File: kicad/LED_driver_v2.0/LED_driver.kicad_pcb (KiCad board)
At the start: 2 copper layers, 39 x 20.5 mm, 11 parts, among them J1 Conn_01x02, J2 Conn_01x02, J3 Conn_01x02, Q1 MMBT3904, Q3 2N7002

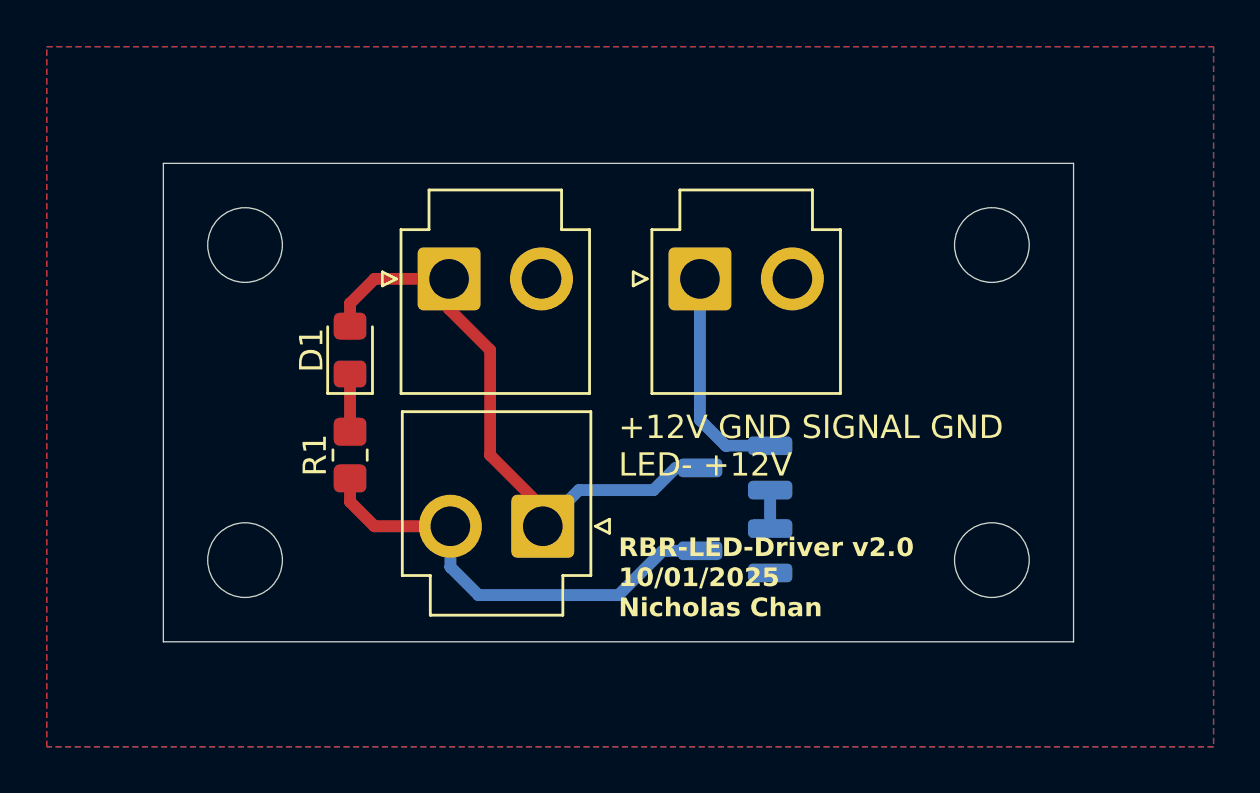
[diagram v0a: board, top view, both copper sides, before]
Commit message: nothing to do
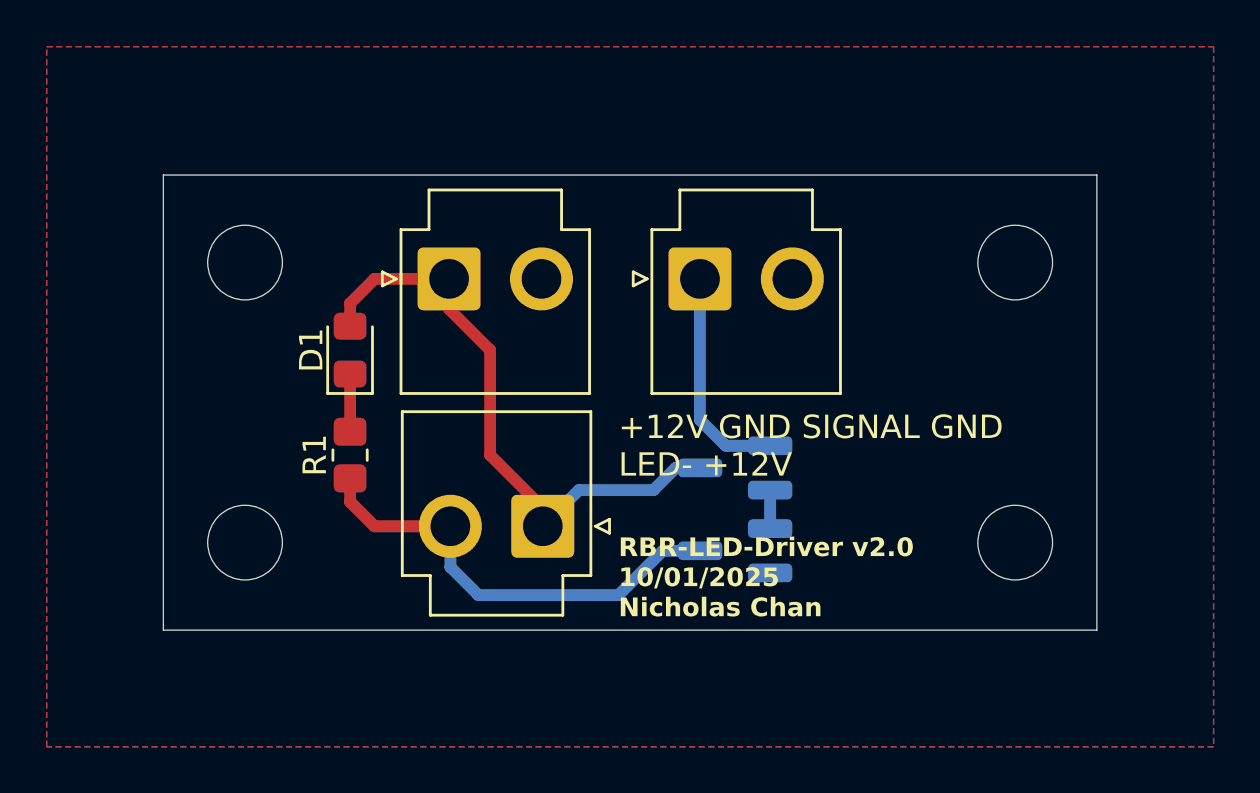
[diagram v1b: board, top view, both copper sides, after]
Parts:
- moved H2 1.25 mm to (136.5, 69.2)
- moved H4 1.25 mm to (136.5, 81.2)
- moved H1 0.75 mm to (103.5, 69.2)
- moved H3 0.75 mm to (103.5, 81.2)
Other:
- board size 39 x 20.5 mm -> 40 x 19.5 mm
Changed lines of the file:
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@@
 	(footprint "MountingHole:MountingHole_3.2mm_M3"
 		(layer "F.Cu")
-		(at 103.5 82)
+		(at 103.5 81.25)
 		(descr "Mounting Hole 3.2mm, no annular, M3")
 		(tags "mounting hole 3.2mm no annular m3")
@@
 	(footprint "MountingHole:MountingHole_3.2mm_M3"
 		(layer "F.Cu")
-		(at 103.5 68.5)
+		(at 103.5 69.25)
 		(descr "Mounting Hole 3.2mm, no annular, M3")
 		(tags "mounting hole 3.2mm no annular m3")
@@
 	(footprint "MountingHole:MountingHole_3.2mm_M3"
 		(layer "F.Cu")
-		(at 135.5 68.5)
+		(at 136.5 69.25)
 		(descr "Mounting Hole 3.2mm, no annular, M3")
 		(tags "mounting hole 3.2mm no annular m3")
@@
 	(footprint "MountingHole:MountingHole_3.2mm_M3"
 		(layer "F.Cu")
-		(at 135.5 82)
+		(at 136.5 81.25)
 		(descr "Mounting Hole 3.2mm, no annular, M3")
 		(tags "mounting hole 3.2mm no annular m3")
@@
 	)
 	(gr_rect
-		(start 100 65)
-		(end 139 85.5)
+		(start 100 65.5)
+		(end 140 85)
 		(stroke
 			(width 0.05)
